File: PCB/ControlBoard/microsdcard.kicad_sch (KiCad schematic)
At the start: 5 parts, among them J4 microSD, Q2 Q_PMOS_GSD

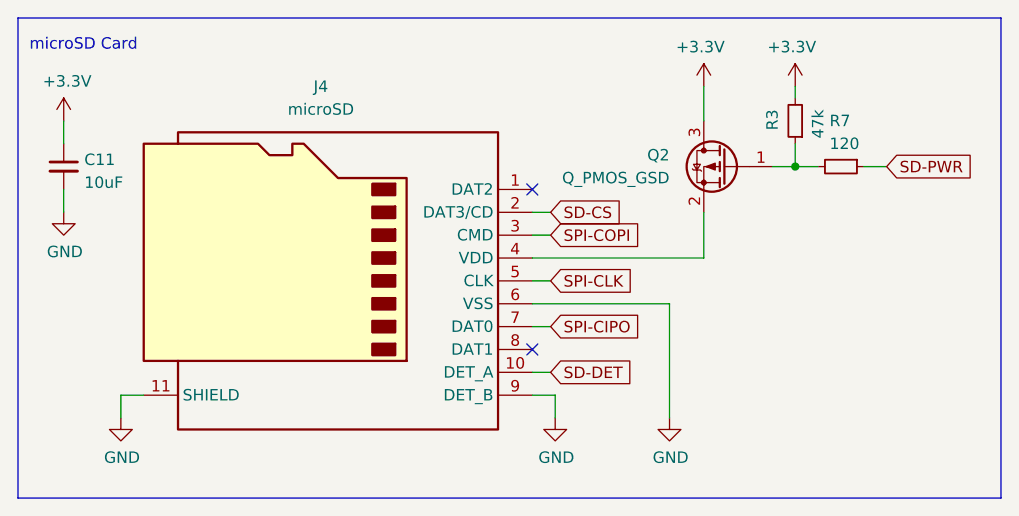
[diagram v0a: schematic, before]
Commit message: First pass of PCB rework.
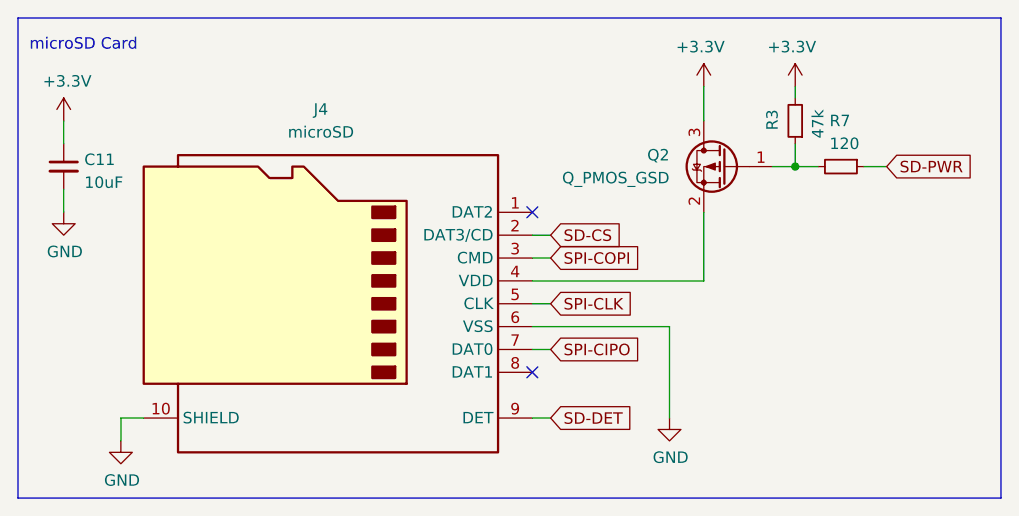
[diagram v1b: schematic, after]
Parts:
- C11: footprint Capacitor_SMD:C_0805_2012Metric -> Capacitor_SMD:C_0603_1608Metric
- J4: footprint (none) -> KTANE:GCT_MEM2075-00-140-01-A; symbol Connector:Micro_SD_Card_Det2 -> Connector:Micro_SD_Card_Det1
- Q2: footprint (none) -> Package_TO_SOT_SMD:SOT-23
- R3, R7: footprint Resistor_SMD:R_0805_2012Metric -> Resistor_SMD:R_0603_1608Metric
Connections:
- net GND: now also J4.10 (SHIELD); no longer J4.11 (SHIELD), J4.9 (DET_B)
- net SD-DET: now also J4.9 (DET); no longer J4.10 (DET_A)
